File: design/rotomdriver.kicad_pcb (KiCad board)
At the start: 2 copper layers, 10 parts, among them P1 SUPPLY, P2 GND, Q1 IRF7749L2TRPBF, Q2 IRF7749L2TRPBF, U1 AD8418

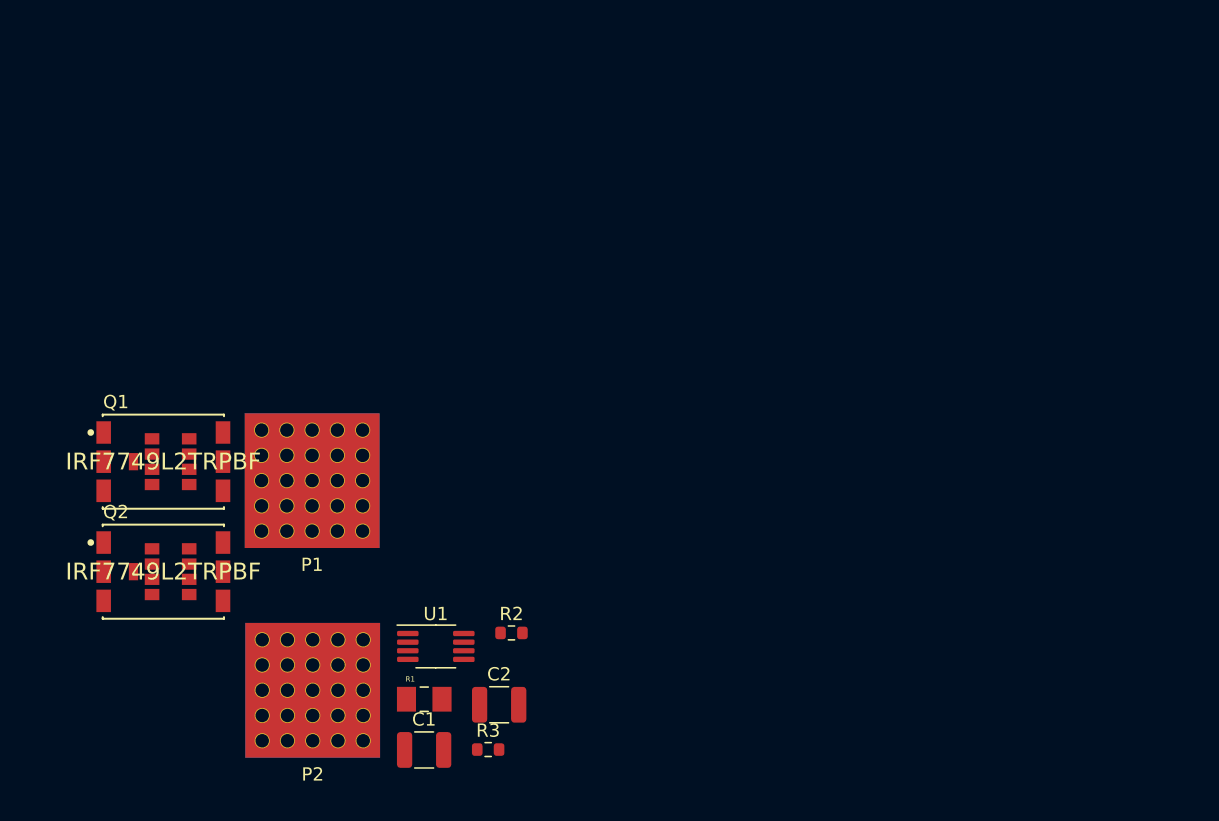
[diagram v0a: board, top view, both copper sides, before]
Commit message: 210104
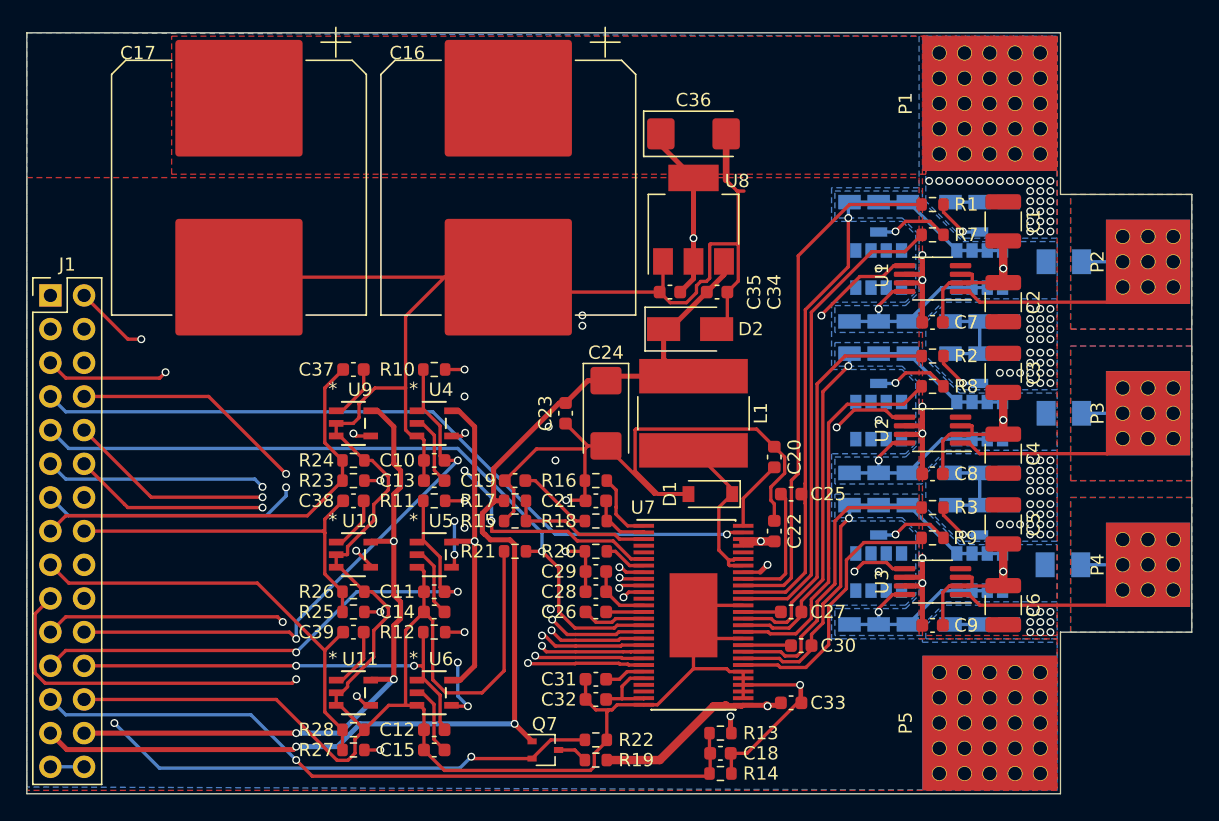
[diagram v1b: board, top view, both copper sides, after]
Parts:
- removed the R3 at (97.5, 83.8)
- added C1: 4.7uF_100V, Capacitor_SMD:C_1210_3225Metric, F.Cu at (136.4, 43.9)
- added C10: 1nF, Capacitor_SMD:C_0603_1608Metric, F.Cu at (93.5, 62.0)
- added C11: 1nF, Capacitor_SMD:C_0603_1608Metric, F.Cu at (93.5, 71.9)
- added C12: 1nF, Capacitor_SMD:C_0603_1608Metric, F.Cu at (93.5, 82.3)
- added C13: 15nF, Capacitor_SMD:C_0603_1608Metric, F.Cu at (93.5, 63.5)
- added C14: 15nF, Capacitor_SMD:C_0603_1608Metric, F.Cu at (93.5, 73.4)
- added C15: 15nF, Capacitor_SMD:C_0603_1608Metric, F.Cu at (93.5, 83.8)
- added C16: 680uF_63V, Capacitor_SMD:CP_Elec_18x22, F.Cu at (99.1, 41.4)
- added C17: 680uF_63V, Capacitor_SMD:CP_Elec_18x22, F.Cu at (78.7, 41.4)
- added C18: 2.2uF, Capacitor_SMD:C_0603_1608Metric, F.Cu at (115.1, 84.1)
- added C19: 6.8nF, Capacitor_SMD:C_0603_1608Metric, F.Cu at (99.6, 63.5)
- added C2: 4.7uF_100V, Capacitor_SMD:C_1210_3225Metric, F.Cu at (136.4, 50.0)
- added C20: 15nF, Capacitor_SMD:C_0603_1608Metric, F.Cu at (119.1, 61.7)
- added C21: 120pF, Capacitor_SMD:C_0603_1608Metric, F.Cu at (105.7, 65.0)
- added C22: 4.7uF_100V, Capacitor_SMD:C_0603_1608Metric, F.Cu at (119.1, 67.3)
- added C23: 2.2uF, Capacitor_SMD:C_0603_1608Metric, F.Cu at (103.4, 58.4)
- added C24: 100uF, Capacitor_Tantalum_SMD:CP_EIA-6032-20_AVX-F, F.Cu at (106.4, 58.4)
- added C25: 220nF, Capacitor_SMD:C_0603_1608Metric, F.Cu at (120.4, 64.5)
- added C26: 22nF, Capacitor_SMD:C_0603_1608Metric, F.Cu at (105.7, 73.4)
- added C27: 220nF, Capacitor_SMD:C_0603_1608Metric, F.Cu at (120.4, 73.4)
- added C28: 2.2uF, Capacitor_SMD:C_0603_1608Metric, F.Cu at (105.7, 71.9)
- added C29: 2.2uF, Capacitor_SMD:C_0603_1608Metric, F.Cu at (105.7, 70.4)
- added C3: 4.7uF_100V, Capacitor_SMD:C_1210_3225Metric, F.Cu at (136.4, 55.4)
- added C30: 220nF, Capacitor_SMD:C_0603_1608Metric, F.Cu at (121.2, 75.9)
- added C31: 2.2uF, Capacitor_SMD:C_0603_1608Metric, F.Cu at (105.7, 78.5)
- added C32: 2.2uF, Capacitor_SMD:C_0603_1608Metric, F.Cu at (105.7, 80.0)
- added C33: 4.7uF_100V, Capacitor_SMD:C_0603_1608Metric, F.Cu at (120.4, 80.3)
- added C34: 2.2uF, Capacitor_SMD:C_0603_1608Metric, F.Cu at (114.8, 49.3)
- added C35: 2.2uF, Capacitor_SMD:C_0603_1608Metric, F.Cu at (111.3, 49.3)
- added C36: 100uF, Capacitor_Tantalum_SMD:CP_EIA-6032-20_AVX-F, F.Cu at (113.0, 37.3)
- added C37: 100nF, Capacitor_SMD:C_0603_1608Metric, F.Cu at (87.4, 55.1)
- added C38: 100nF, Capacitor_SMD:C_0603_1608Metric, F.Cu at (87.4, 65.0)
- added C39: 100nF, Capacitor_SMD:C_0603_1608Metric, F.Cu at (87.4, 74.9)
- added C4: 4.7uF_100V, Capacitor_SMD:C_1210_3225Metric, F.Cu at (136.4, 61.5)
- added C7: 2.2uF, Capacitor_SMD:C_0603_1608Metric, F.Cu at (131.1, 51.6)
- added C8: 2.2uF, Capacitor_SMD:C_0603_1608Metric, F.Cu at (131.1, 63.0)
- added C9: 2.2uF, Capacitor_SMD:C_0603_1608Metric, F.Cu at (131.1, 74.4)
- added D1: DIODE, Diode_SMD:D_SOD-123, F.Cu at (114.3, 64.5)
- added D2: TVS 5V, Diode_SMD:D_SMA, F.Cu at (112.8, 52.1)
- added J1: Conn_01x30_Male, Connector_PinHeader_2.54mm:PinHeader_2x15_P2.54mm_Vertical, F.Cu at (64.5, 49.5)
- added L1: 22uH, Inductor_SMD:L_Bourns-SRN8040_8x8.15mm, F.Cu at (113.0, 58.4)
- added P3: PH_B, PADS:HighCurrent_WithHoles_250mils, F.Cu at (147.3, 58.4)
- added P4: PH_C, PADS:HighCurrent_WithHoles_250mils, F.Cu at (147.3, 69.8)
- added P5: GND, PADS:HighCurrent_WithHoles_400mils, F.Cu at (135.4, 81.8)
- added Q1: IRF7749L2TRPBF, IRF7749L2TRPBF:Infineon-IRF7749L2TRPBF-0-0-0, B.Cu at (134.6, 47.0)
- added Q4: IRF7749L2TRPBF, IRF7749L2TRPBF:Infineon-IRF7749L2TRPBF-0-0-0, B.Cu at (127.0, 47.0)
- added Q5: IRF7749L2TRPBF, IRF7749L2TRPBF:Infineon-IRF7749L2TRPBF-0-0-0, B.Cu at (127.0, 58.4)
- added Q6: IRF7749L2TRPBF, IRF7749L2TRPBF:Infineon-IRF7749L2TRPBF-0-0-0, B.Cu at (127.0, 69.8)
- added Q7: DMN62D0UW-7, Package_TO_SOT_SMD:SOT-323_SC-70, F.Cu at (101.9, 83.8)
- added R10: 1k, Resistor_SMD:R_0603_1608Metric, F.Cu at (93.5, 55.1)
- added R11: 1k, Resistor_SMD:R_0603_1608Metric, F.Cu at (93.5, 65.0)
- added R12: 1k, Resistor_SMD:R_0603_1608Metric, F.Cu at (93.5, 74.9)
- added R13: NTC 10k, Resistor_SMD:R_0603_1608Metric, F.Cu at (115.1, 82.5)
- added R14: 10k, Resistor_SMD:R_0603_1608Metric, F.Cu at (115.1, 85.6)
- added R15: 3.3k, Resistor_SMD:R_0603_1608Metric, F.Cu at (99.6, 66.5)
- added R16: 220k, Resistor_SMD:R_0603_1608Metric, F.Cu at (105.7, 63.5)
- added R17: 18k, Resistor_SMD:R_0603_1608Metric, F.Cu at (99.6, 65.0)
- added R18: 15k, Resistor_SMD:R_0603_1608Metric, F.Cu at (105.7, 66.5)
- added R19: 39k, Resistor_SMD:R_0603_1608Metric, F.Cu at (105.7, 84.6)
- added R2: 4.7R, Resistor_SMD:R_0603_1608Metric, F.Cu at (131.1, 54.1)
- added R20: 10k, Resistor_SMD:R_0603_1608Metric, F.Cu at (105.7, 68.8)
- added R21: 10k, Resistor_SMD:R_0603_1608Metric, F.Cu at (99.6, 68.8)
- added R22: 2k2, Resistor_SMD:R_0603_1608Metric, F.Cu at (105.7, 83.1)
- added R23: 39k, Resistor_SMD:R_0603_1608Metric, F.Cu at (87.4, 63.5)
- added R24: 2k2, Resistor_SMD:R_0603_1608Metric, F.Cu at (87.4, 62.0)
- added R25: 39k, Resistor_SMD:R_0603_1608Metric, F.Cu at (87.4, 73.4)
- added R26: 2k2, Resistor_SMD:R_0603_1608Metric, F.Cu at (87.4, 71.9)
- added R27: 39k, Resistor_SMD:R_0603_1608Metric, F.Cu at (87.4, 83.8)
- added R28: 2k2, Resistor_SMD:R_0603_1608Metric, F.Cu at (87.4, 82.3)
- added R4: 0.0005R, HighCurrentShunt:RESC3216X105N, B.Cu at (141.0, 47.0)
- added R5: 0.0005R, HighCurrentShunt:RESC3216X105N, B.Cu at (141.0, 58.4)
- added R6: 0.0005R, HighCurrentShunt:RESC3216X105N, B.Cu at (140.9, 69.8)
- added R7: 4.7R, Resistor_SMD:R_0603_1608Metric, F.Cu at (131.1, 45.0)
- added R8: 4.7R, Resistor_SMD:R_0603_1608Metric, F.Cu at (131.1, 56.4)
- added R9: 4.7R, Resistor_SMD:R_0603_1608Metric, F.Cu at (131.1, 67.8)
- added U1: AD8418, Package_SO:MSOP-8_3x3mm_P0.65mm, F.Cu at (131.1, 48.3)
- added U10: M74VHC1GT66DTT1G, AnalogSwitch:M74VHC1GT66DTT1G, F.Cu at (87.4, 69.1)
- added U11: M74VHC1GT66DTT1G, AnalogSwitch:M74VHC1GT66DTT1G, F.Cu at (87.4, 79.5)
- added U2: AD8418, Package_SO:MSOP-8_3x3mm_P0.65mm, F.Cu at (131.1, 59.7)
- added U4: M74VHC1GT66DTT1G, AnalogSwitch:M74VHC1GT66DTT1G, F.Cu at (93.5, 59.2)
- added U5: M74VHC1GT66DTT1G, AnalogSwitch:M74VHC1GT66DTT1G, F.Cu at (93.5, 69.1)
- added U6: M74VHC1GT66DTT1G, AnalogSwitch:M74VHC1GT66DTT1G, F.Cu at (93.5, 79.5)
- added U7: DRV8301DCAR, Package_SO:HTSSOP-56-1EP_6.1x14mm_P0.5mm_EP3.61x6.35mm, F.Cu at (113.0, 73.7)
- added U8: TC2117-3.3VDBTR, Package_TO_SOT_SMD:SOT-223-3_TabPin2, F.Cu at (113.0, 43.8)
- added U9: M74VHC1GT66DTT1G, AnalogSwitch:M74VHC1GT66DTT1G, F.Cu at (87.4, 59.2)
- P2: value GND -> PH_A; footprint PADS:HighCurrent_WithHoles_400mils -> PADS:HighCurrent_WithHoles_250mils
- Q2: moved to B.Cu
- Q3: renamed from Q1; moved to B.Cu
- R1: value 0.0005R -> 4.7R; footprint HighCurrentShunt:RESC3216X105N -> Resistor_SMD:R_0603_1608Metric
- moved P2 70.8 mm to (147.3, 47.0)
- moved Q2 62.7 mm to (134.6, 58.4), turned to 270 degrees
- moved Q3 62.1 mm to (134.6, 69.8), turned to 270 degrees
- moved P1 58.5 mm to (135.4, 35.1)
- moved R1 53.5 mm to (131.1, 42.7), turned to 180 degrees
- moved C5 46.9 mm to (136.4, 66.8), turned to 270 degrees
- moved C6 38.8 mm to (136.4, 72.9), turned to 90 degrees
- moved U3 37.8 mm to (131.1, 71.1), turned to 180 degrees
- moved R3 33.1 mm to (131.1, 65.5), turned to 180 degrees
- renumbered C1 to C5, C2 to C6, R2 to R3, U1 to U3
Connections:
- C5 pad 1: /power/SUPPLY -> SUPPLY
- C6 pad 1: /power/SUPPLY -> SUPPLY
- P1 pad 1: /power/SUPPLY -> SUPPLY
- P2 pad 1: GND -> Net-(P2-Pad1)
- Q2 pad 1: /power/SH_C -> SUPPLY
- Q2 pad 10: GND -> /drv8301/SH_B
- Q2 pad 11: GND -> /drv8301/SH_B
- Q2 pad 2: GND -> /drv8301/SH_B
- Q2 pad 3: GND -> /drv8301/SH_B
- Q2 pad 4: /power/SH_C -> SUPPLY
- Q2 pad 5: GND -> /drv8301/SH_B
- Q2 pad 6: GND -> /drv8301/SH_B
- Q2 pad 8: GND -> /drv8301/SH_B
- Q2 pad 9: GND -> /drv8301/SH_B
- Q3 pad 1: /power/SUPPLY -> SUPPLY
- Q3 pad 10: Net-(Q1-Pad10) -> /drv8301/SH_C
- Q3 pad 11: Net-(Q1-Pad11) -> /drv8301/SH_C
- Q3 pad 2: /power/SH_C -> /drv8301/SH_C
- Q3 pad 3: Net-(Q1-Pad3) -> /drv8301/SH_C
- Q3 pad 4: /power/SUPPLY -> SUPPLY
- Q3 pad 5: Net-(Q1-Pad5) -> /drv8301/SH_C
- Q3 pad 6: Net-(Q1-Pad6) -> /drv8301/SH_C
- Q3 pad 8: Net-(Q1-Pad8) -> /drv8301/SH_C
- Q3 pad 9: Net-(Q1-Pad9) -> /drv8301/SH_C
- R1 pad 1: Net-(R1-Pad1) -> Net-(Q1-Pad7)
- R1 pad 2: /power/SH_C -> /drv8301/GH_A
- R3 pad 2: /power/GH_C -> /drv8301/GH_C
- U3 pad 1: Net-(R1-Pad1) -> Net-(P4-Pad1)
- U3 pad 2: Net-(U1-Pad2) -> GND
- U3 pad 3: Net-(U1-Pad3) -> GND
- U3 pad 5: Net-(U1-Pad5) -> /power/C_C
- U3 pad 6: Net-(U1-Pad6) -> +3V3
- U3 pad 7: Net-(U1-Pad7) -> +3V3
- U3 pad 8: /power/SH_C -> /drv8301/SH_C
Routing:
- net GND: track 0.00 -> 402.6 mm, vias 0 -> 9
- net +3V3: track 0.00 -> 204.8 mm, vias 0 -> 13
- net /SH_A: track 0.00 -> 110.0 mm, vias 0 -> 5
- net /drv8301/SH_B: track 0.00 -> 98.9 mm, vias 0 -> 5
- net +5V: track 0.00 -> 90.8 mm, vias 0 -> 2
- net /drv8301/SH_C: track 0.00 -> 90.1 mm, vias 0 -> 3
- net /drv8301/INH_A: track 0.00 -> 67.0 mm, vias 0 -> 1
- net /drv8301/INL_B: track 0.00 -> 65.4 mm, vias 0 -> 2
- net /drv8301/INH_C: track 0.00 -> 64.9 mm, vias 0 -> 1
- net /drv8301/INH_B: track 0.00 -> 63.9 mm, vias 0 -> 2
- net /drv8301/INL_A: track 0.00 -> 62.7 mm, vias 0 -> 1
- net /drv8301/INL_C: track 0.00 -> 61.2 mm, vias 0 -> 1
- net /power/CURR_FILTER: track 0.00 -> 58.2 mm, vias 0 -> 6
- net /EN_BUCK: track 0.00 -> 56.6 mm, vias 0 -> 1
- net /drv8301/SENS_FILTERED: track 0.00 -> 55.7 mm, vias 0 -> 4
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- added copper zone on B.Cu, net /SH_A
- added copper zone on B.Cu, net /drv8301/SH_B
- added copper zone on B.Cu, net /drv8301/SH_C
- added copper zone on B.Cu, net GND
- added copper zone on F.Cu, net GND
- added copper zone on In1_G.Cu, net GND
- added copper zone on In2_V.Cu, net GND
- added copper zone on B.Cu, net Net-(P2-Pad1)
- added copper zone on F.Cu, net Net-(P2-Pad1)
- added copper zone on B.Cu, net Net-(P3-Pad1)
- added copper zone on F.Cu, net Net-(P3-Pad1)
- added copper zone on B.Cu, net Net-(P4-Pad1)
- added copper zone on F.Cu, net Net-(P4-Pad1)
- added copper zone on B.Cu, net SUPPLY
- added copper zone on F.Cu, net SUPPLY
- added copper zone on In2_V.Cu, net SUPPLY
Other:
- board outline added: 87.9 x 57.4 mm
- copper layers 2 -> 4
- net class Default: clearance 0.2 -> 0.18; trace_width 0.25 -> 0.254; via_dia 0.8 -> 0.6
- net class Pwr added: clearance 0.2, trace_width 0.635, via_dia 0.6, via_drill 0.4
- net class Vcc added: clearance 0.2, trace_width 0.381, via_dia 0.6, via_drill 0.4
- rule trace_clearance: 0.2 -> 0.18
- board text added: "Rotom Driver 2021-01-04"
